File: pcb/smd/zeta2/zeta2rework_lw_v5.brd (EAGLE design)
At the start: 80.3 x 43.2 mm, 104 parts, among them IC1 MAX6520, IC2 L293DD, IC3 L293DD, Q12 8MHz, U1 MPU-6050, U2 INA219, U5 DS18B20U+

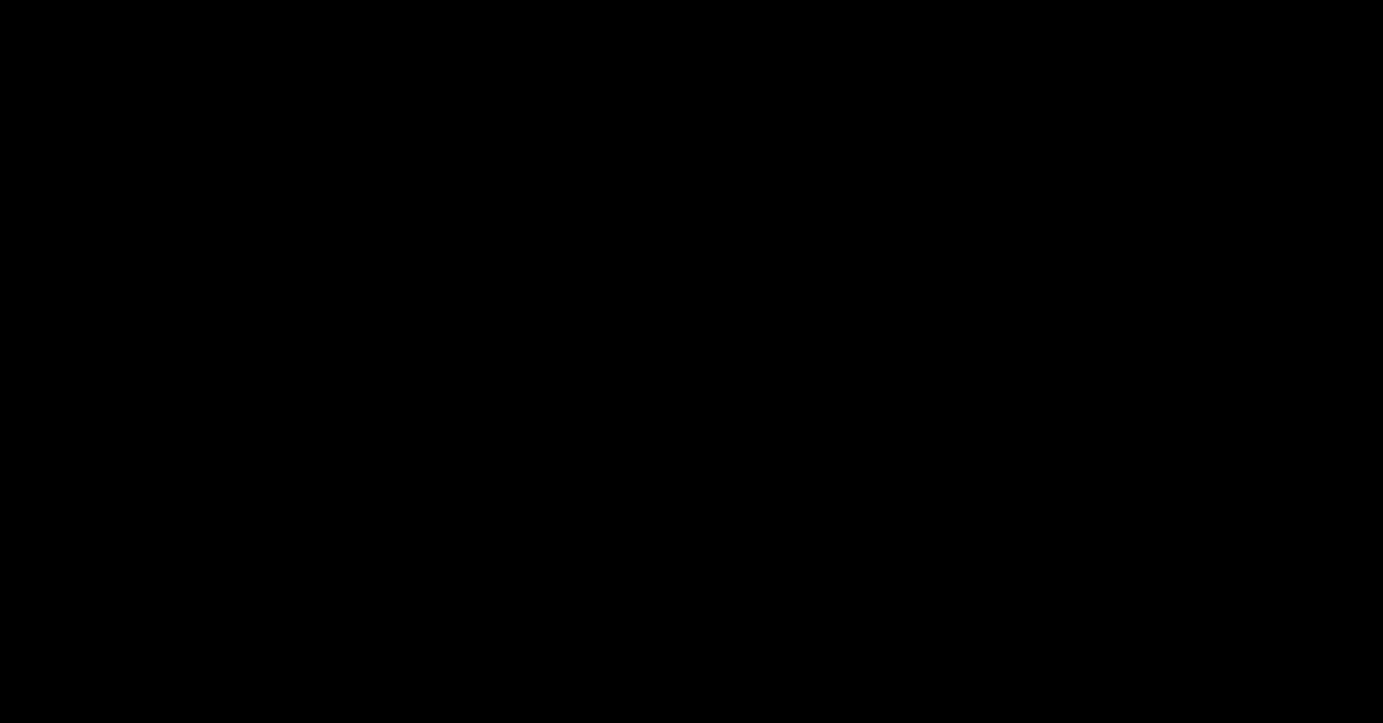
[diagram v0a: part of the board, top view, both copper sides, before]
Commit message: finished pcb
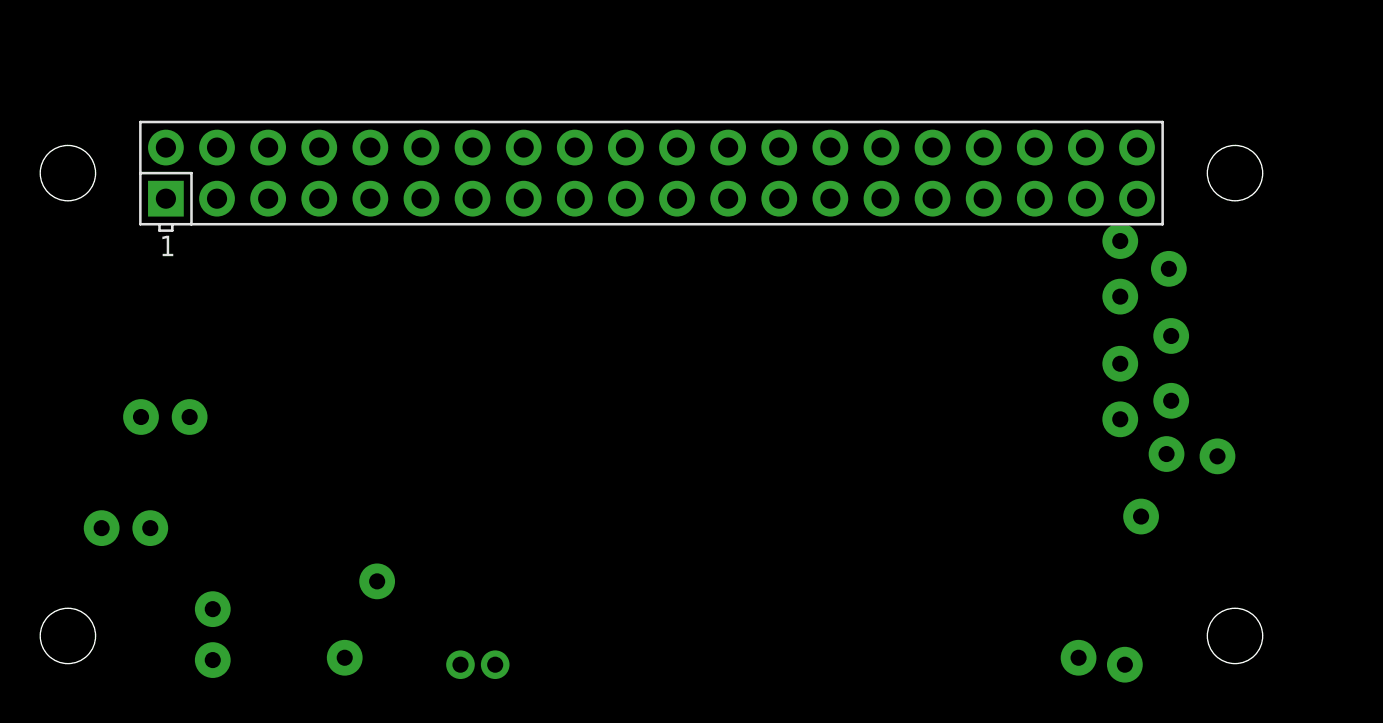
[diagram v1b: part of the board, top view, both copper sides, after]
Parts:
- added U$2: RPI-ZERO, rpi-zero:RASP_PI_ZERO_BOARD_FULL
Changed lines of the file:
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@@
 <drawing>
 <settings>
-<setting alwaysvectorfont="yes"/>
+<setting alwaysvectorfont="no"/>
 <setting verticaltext="up"/>
 </settings>
@@
 <attribute name="SPICEPREFIX" value="C" x="71.12" y="29.21" size="1.778" layer="27" display="off"/>
 </element>
+<element name="U$2" library="rpi-zero" package="RASP_PI_ZERO_BOARD_FULL" value="RPI-ZERO" x="-10.795" y="-84.455"/>
 </elements>
 <signals>
